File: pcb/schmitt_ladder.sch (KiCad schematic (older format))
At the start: 21 parts, among them U1 OPA2156xDGK, U2 OPA2156xDGK, U3 OPA2156xDGK

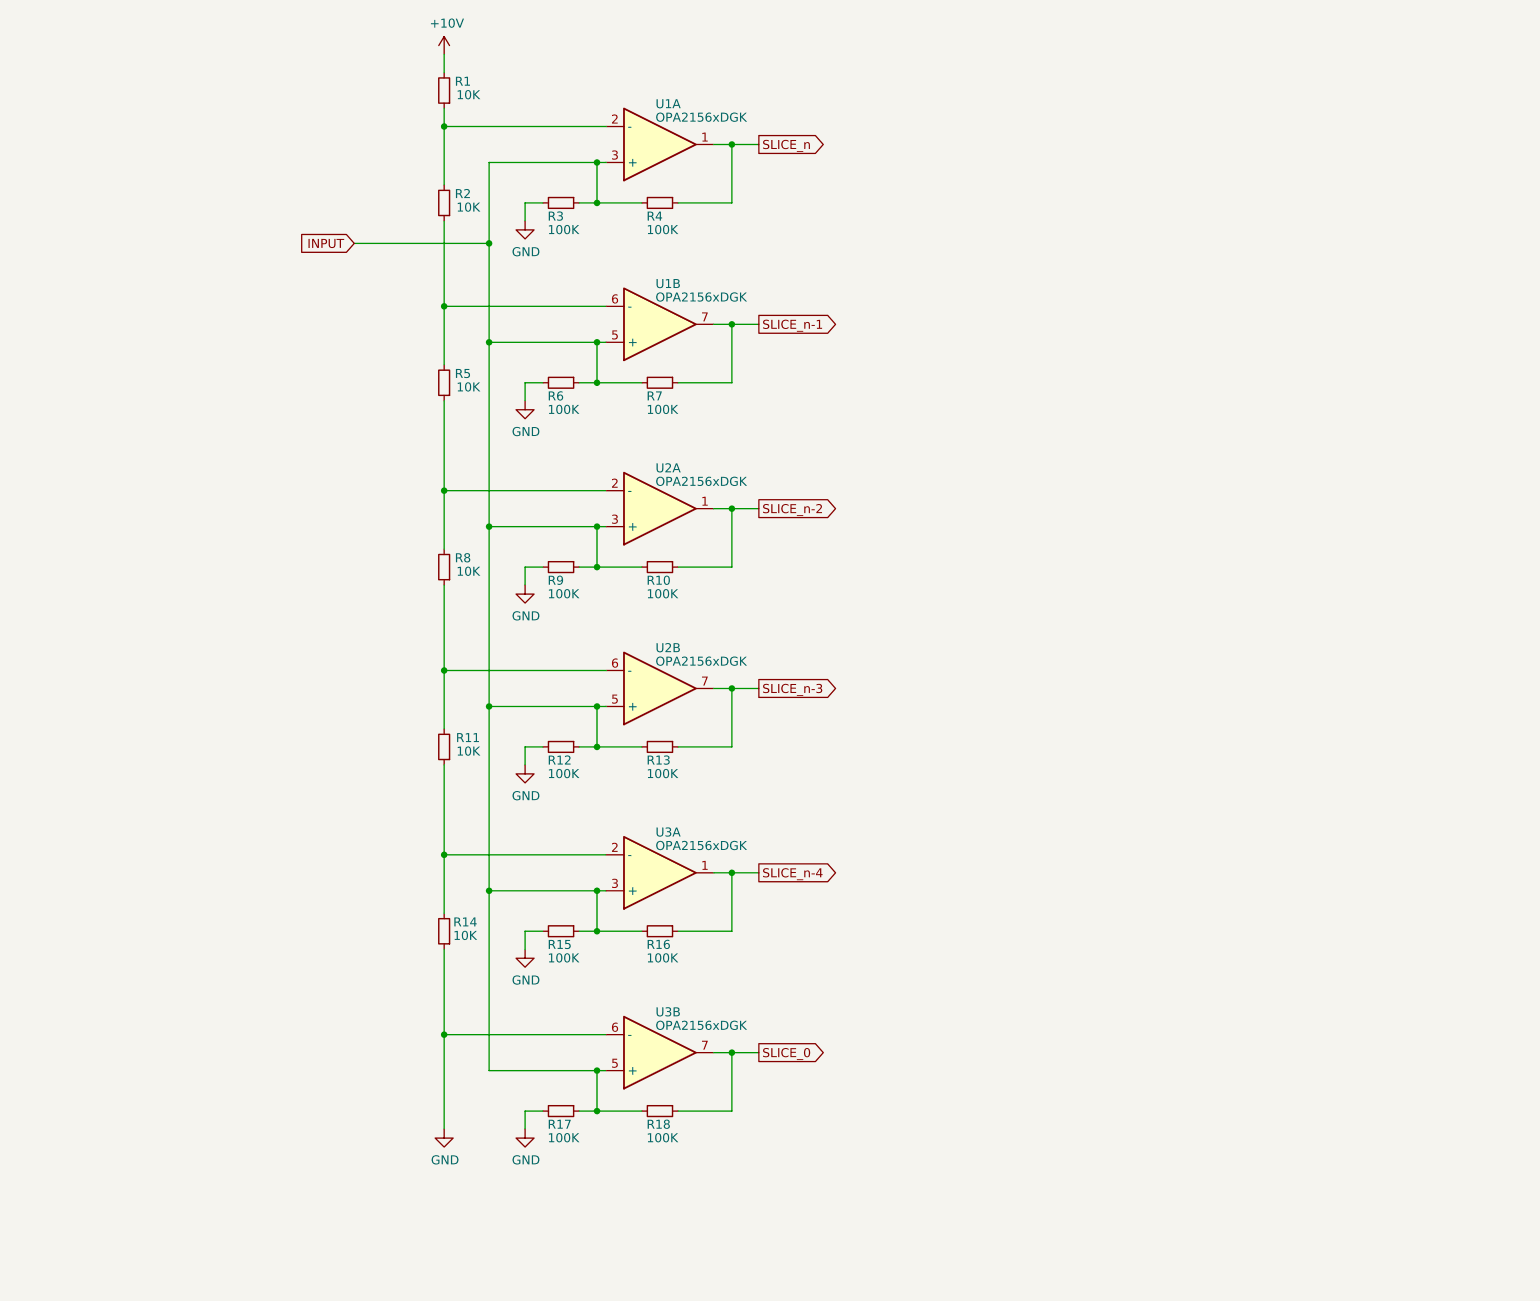
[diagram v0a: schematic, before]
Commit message: working on algorithm 4
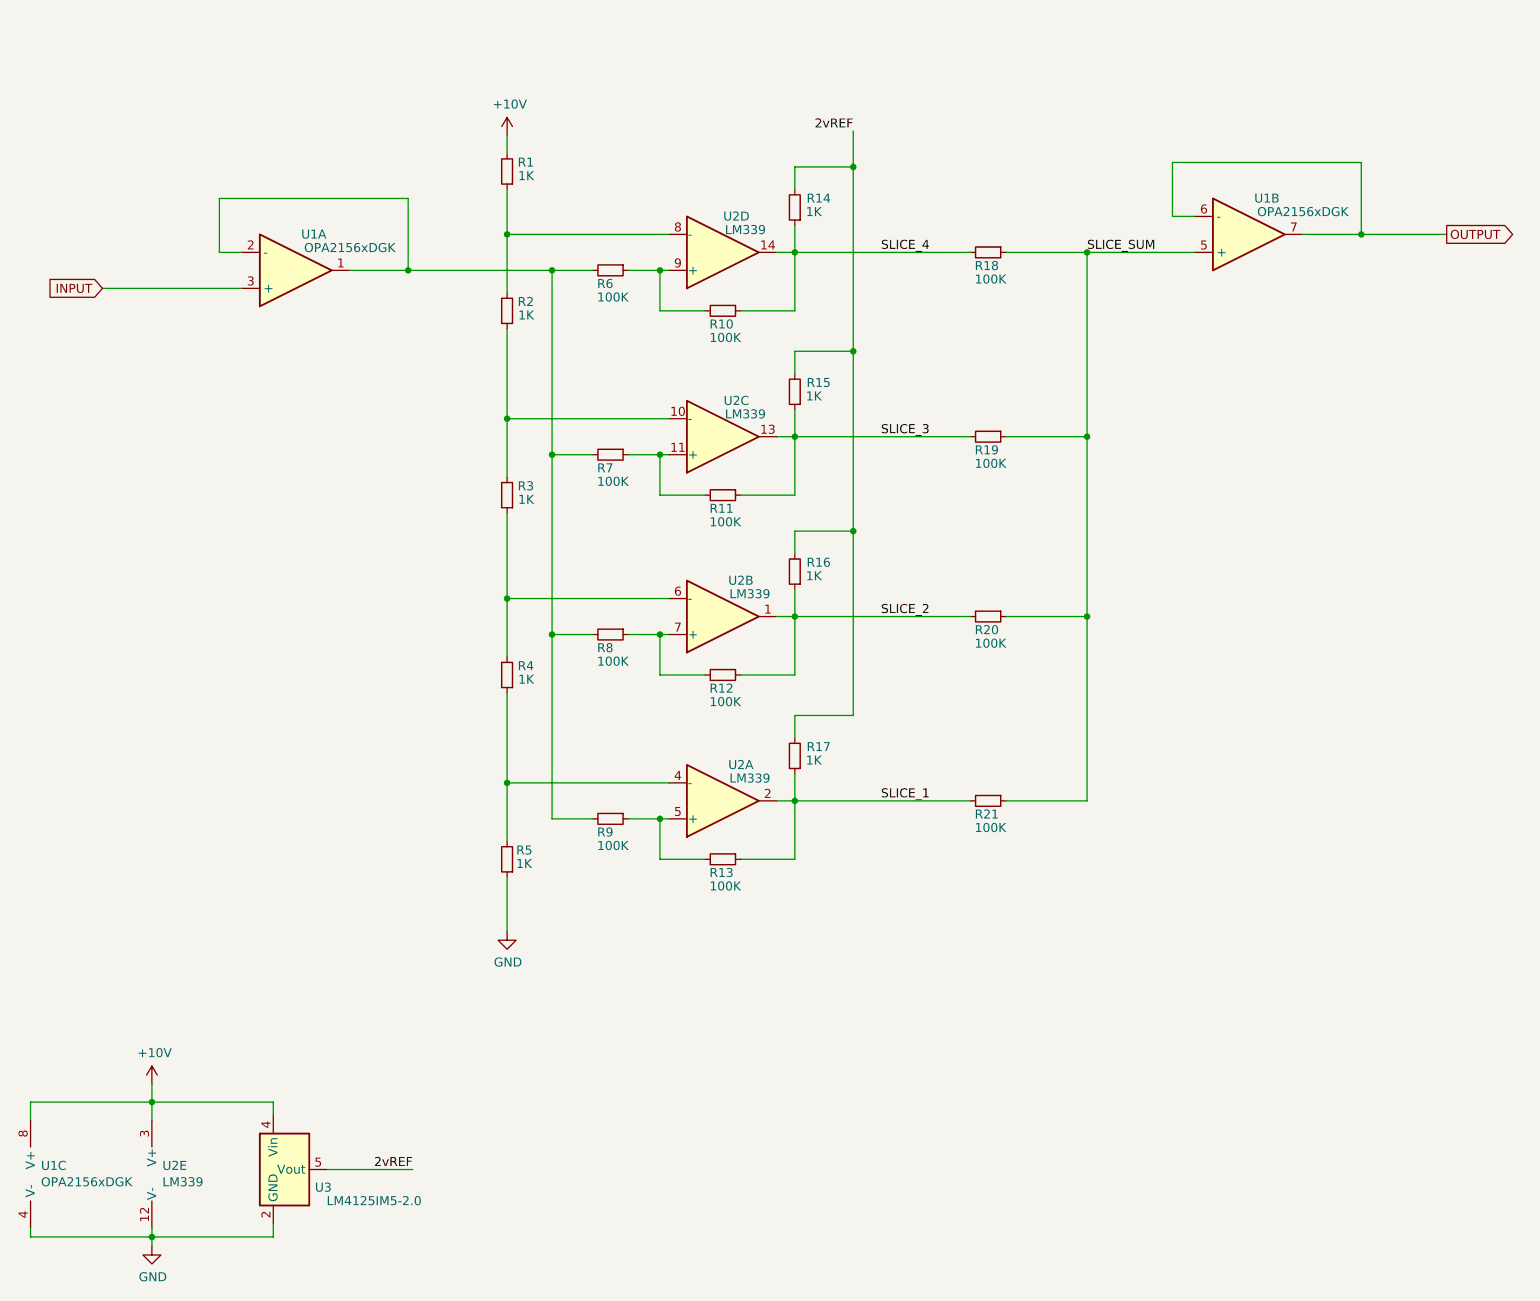
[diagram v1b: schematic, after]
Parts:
- removed R2: 10K, Resistor_SMD:R_0805_2012Metric, symbol schmitt_ladder-rescue:R_Small-device-2019-04-06_Range_Slicer_PCB-rescue-Range_S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
- removed R3, R4: 100K, Resistor_SMD:R_0805_2012Metric, symbol schmitt_ladder-rescue:R_Small-device-2019-04-06_Range_Slicer_PCB-rescue-Range_S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
- removed U2, U3: OPA2156xDGK, Package_SO:VSSOP-8_3.0x3.0mm_P0.65mm, symbol Amplifier_Operational:OPA2156xDGK
- added R14, R15, R16: 1K, Resistor_SMD:R_0805_2012Metric, symbol schmitt_ladder-rescue:R_Small-device-2019-04-06_Range_Slicer_PCB-rescue-Range_S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
- added R19, R20, R21: 100K, Resistor_SMD:R_0805_2012Metric, symbol schmitt_ladder-rescue:R_Small-device-2019-04-06_Range_Slicer_PCB-rescue-Range_S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
- added unit 3 of U1
- added U2: LM339, symbol Comparator:LM339
- added U3: LM4125IM5-2.0, Package_TO_SOT_SMD:SOT-23-5, symbol Reference_Voltage:LM4125IM5-2.0
- R1: value 10K -> 1K
- R17: value 100K -> 1K
- R2: renamed from R5; value 10K -> 1K
- R3: renamed from R8; value 10K -> 1K
- R4: renamed from R11; value 10K -> 1K
- R5: renamed from R14; value 10K -> 1K
- renumbered R7 to R10, R10 to R11, R13 to R12, R16 to R13, R9 to R7, R12 to R8, R15 to R9
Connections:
- net +10V: now also U1.8 (V+), U2.3 (V+), U3.4 (Vin)
- net GND: now also U1.4 (V-), U2.12 (V-), U3.2 (GND); no longer R17.2, R6.2, R7.2, R8.2, R9.2
- net INPUT: no longer R10.2, R11.2, R12.2, R13.2, R17.1, R18.2, R6.1, R7.1, R8.1, R9.1, U1.5 (+)
- net at R1.1: now also R2.2, U2.8 (-); no longer U1.2 (-)
- net OUTPUT: now reaches U1.6 (-)
- net OUTPUT: now also U1.7; no longer R2.2
- net at R2.1, R3.2: now also U2.10 (-)
- net at R3.1, R4.2: now also U2.6 (-)
- net at R4.1, R5.2: now also U2.4 (-)
- net SLICE_0 renamed SLICE_SUM
- net SLICE_SUM: now also U1.5 (+), R19.1, R20.1, R21.1
- net SLICE_n: no longer names the net of U1.1
- net SLICE_n: now also R6.2, R7.2, R8.2, R9.2, U1.2 (-)
- net SLICE_n-1 renamed SLICE_4
- net SLICE_4: now also R18.2, R14.1, U2.14; no longer U1.7
- net SLICE_n-2 renamed SLICE_3
- net SLICE_3: now also R15.1, R19.2, U2.13
- net SLICE_n-3 renamed SLICE_2
- net SLICE_2: now also R16.1, R20.2, U2.1
- net SLICE_n-4 renamed SLICE_1
- net SLICE_1: now also R17.1, R21.2, U2.2
- new net: R13.2, R9.1, U2.5 (+)
- new net: R12.2, R8.1, U2.7 (+)
- new net: R11.2, R7.1, U2.11 (+)
- new net: R10.2, R6.1, U2.9 (+)
- new net 2vREF: R14.2, R15.2, R16.2, R17.2, U3.5 (Vout)
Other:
- moved on the sheet: R1, R10, R11, R12, R13, R2, R3, R4, R5, R6, R7, R8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
